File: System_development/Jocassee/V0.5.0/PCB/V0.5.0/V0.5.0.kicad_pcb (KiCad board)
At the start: 2 copper layers, 32.6 x 97.2 mm, 16 parts, among them U1 water_Battery, U2 SD, U3 switch, U4 Sensor, U5 Sensor, U6 DS3231M, U7 Sensor, U8 Temp

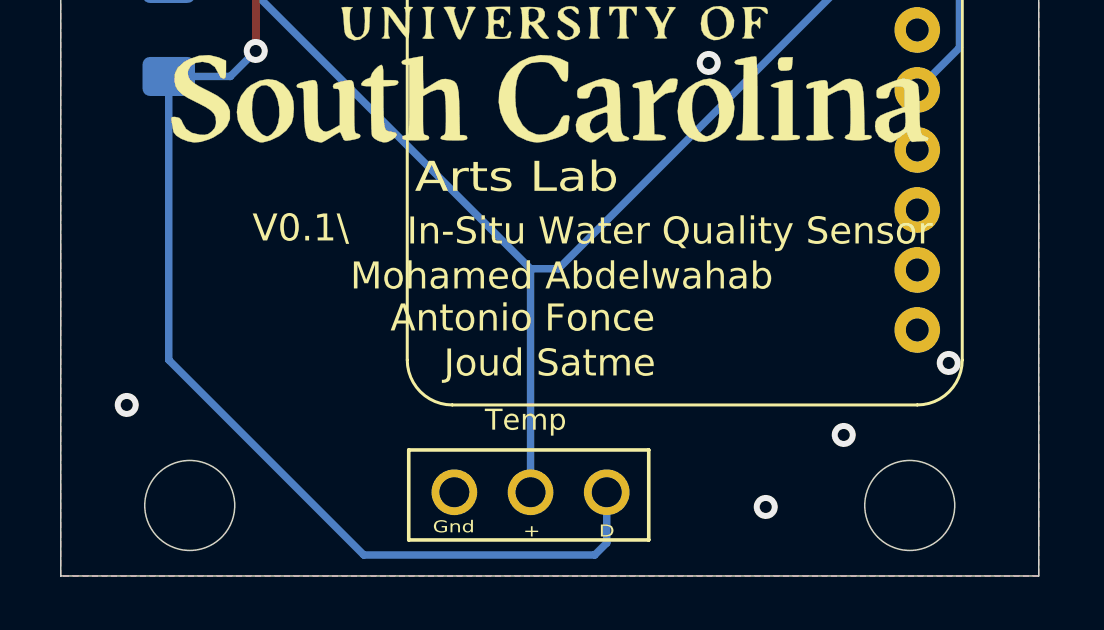
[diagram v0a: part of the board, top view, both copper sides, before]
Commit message: V0.5.0 PCB Update
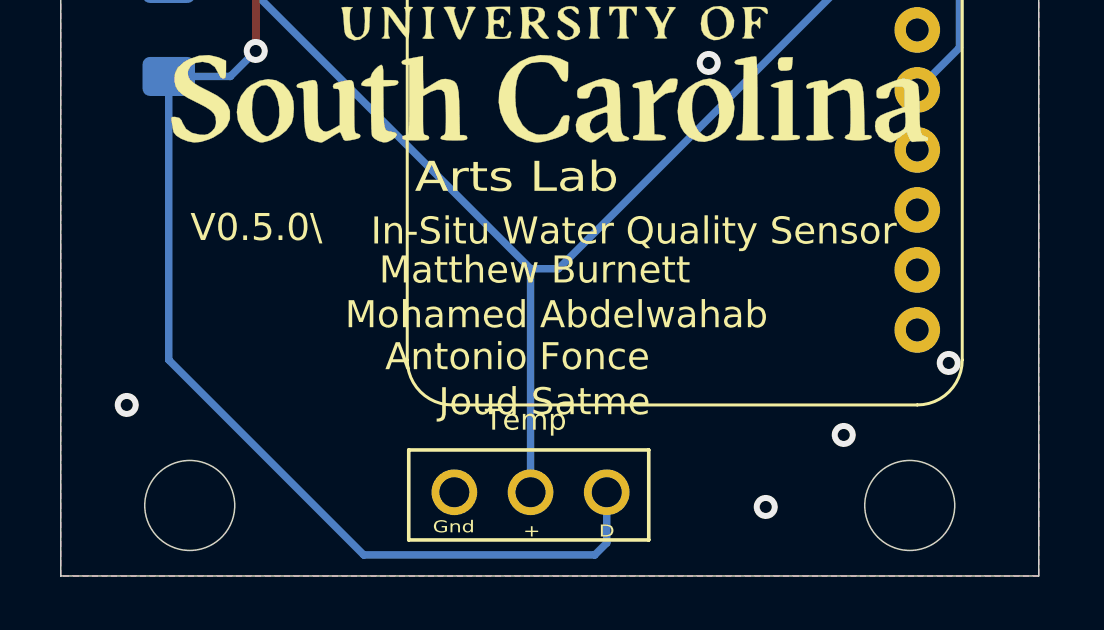
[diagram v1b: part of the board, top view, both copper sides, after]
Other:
- board text added: "Matthew Burnett"
- board text added: "V0.5.0\"
- board text removed: "V0.1\"
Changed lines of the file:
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@@
 	)
 	(gr_text "Joud Satme"
-		(at 113.5 117.1 0)
+		(at 113.324878 118.39123 0)
+		(layer "F.SilkS")
+		(effects
+			(font
+				(size 0.9 0.9)
+				(thickness 0.2)
+			)
+		)
+	)
+	(gr_text "Matthew Burnett"
+		(at 113 114 0)
 		(layer "F.SilkS")
 		(effects
@@
 	)
 	(gr_text "In-Situ Water Quality Sensor"
-		(at 117.5 112.7 0)
+		(at 116.3 112.7 0)
 		(layer "F.SilkS")
 		(effects
@@
 		)
 	)
-	(gr_text "V0.1\\"
-		(at 105.2 112.6 0)
+	(gr_text "V0.5.0\\"
+		(at 103.721423 112.584747 0)
 		(layer "F.SilkS")
 		(effects
@@
 	)
 	(gr_text "Antonio Fonce"
-		(at 112.6 115.6 0)
+		(at 112.424878 116.89123 0)
 		(layer "F.SilkS")
 		(effects
@@
 	)
 	(gr_text "Mohamed Abdelwahab"
-		(at 113.9 114.2 0)
+		(at 113.724878 115.49123 0)
 		(layer "F.SilkS")
 		(effects
